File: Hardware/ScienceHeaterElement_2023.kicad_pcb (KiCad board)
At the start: 2 copper layers, 61.3 x 44.1 mm, 16 parts, among them Q1 BUK7M6R3-40EX, U1 LMT85DCK

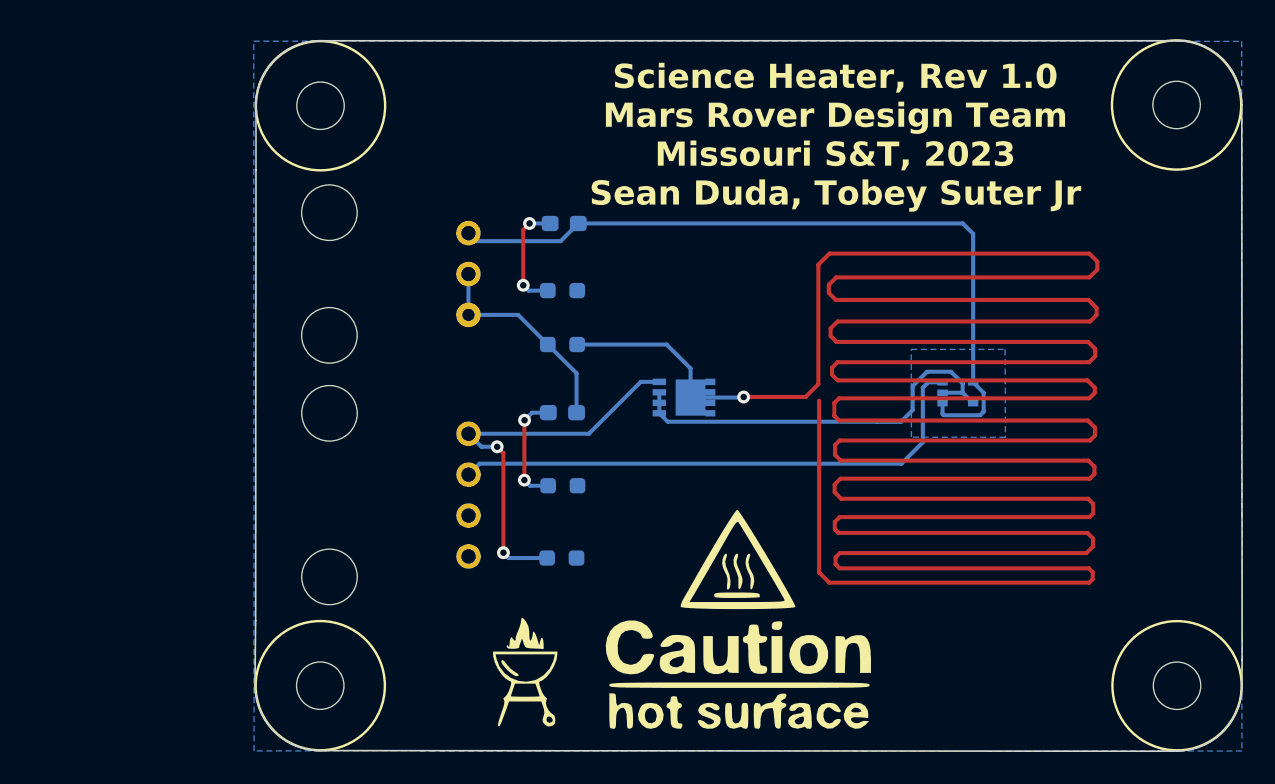
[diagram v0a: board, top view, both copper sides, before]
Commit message: Updated layout for order
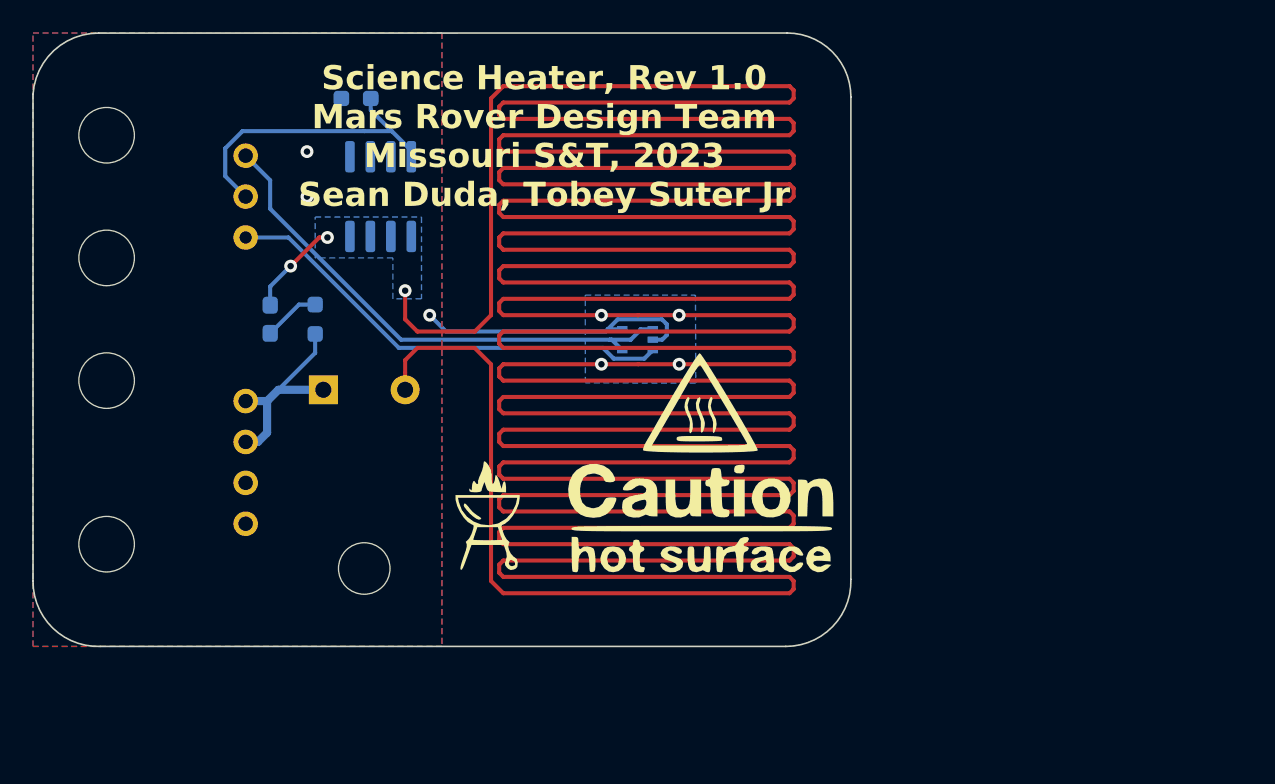
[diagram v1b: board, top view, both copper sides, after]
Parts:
- removed D2: Green, LED_SMD:LED_0603_1608Metric_Pad1.05x0.95mm_HandSolder
- removed R4: 4.7k, Resistor_SMD:R_0603_1608Metric_Pad0.98x0.95mm_HandSolder
- removed REF** (x4): 4_40_Hole, MRDT_Drill_Holes:4_40_Hole_Corner
- added G***: LOGO, LOGO, B.Cu at (105.2, 61.5)
- added G***: LOGO, LOGO, B.Cu at (91.9, 58.4)
- D1: value Green -> ORANGE
- Q1: value BUK7M6R3-40EX -> Si4162DY; footprint Package_TO_SOT_SMD:LFPAK33 -> Package_SO:SOIC-8_3.9x4.9mm_P1.27mm
- R1: value 2 -> 7.5; footprint Resistor_SMD:R_0603_1608Metric_Pad0.98x0.95mm_HandSolder -> Package_TO_SOT_THT:TO-126-2_Horizontal_TabDown
- R2: value 300 -> 1000
- R3: value 1k -> 4.7k
- moved R3 27.3 mm to (77.2, 35.8), turned to 180 degrees
- moved Q1 22.6 mm to (78.7, 41.9), turned to -90 degrees
- moved U1 20.2 mm to (94.7, 50.8), turned to 180 degrees
- moved D1 19.2 mm to (71.9, 49.5), turned to -90 degrees
- moved R2 15.5 mm to (74.7, 49.5), turned to 90 degrees
- moved R1 15.1 mm to (75.2, 53.9)
- moved Conn1 14.7 mm to (70.4, 39.4)
- moved Conn2 14.0 mm to (70.4, 54.6)
- moved G*** 10.00 mm to (98.6, 58.4)
- moved G*** 10.00 mm to (85.3, 61.5)
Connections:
- Conn1 pad 2: +12V -> Gate_Driving_Pin
- Conn1 pad 3: +12V -> Temp_Sense
- Conn2 pad 1: Gate_Driving_Pin -> +12V
- Conn2 pad 2: Temp_Sense -> +12V
- D1 pad 1: Net-(D1-K) -> /Heater_Trace
- D1 pad 2: +3.3V -> Net-(D1-A)
- R2 pad 1: Net-(D1-K) -> +12V
- R2 pad 2: GND -> Net-(D1-A)
- R3 pad 1: Net-(D2-K) -> Gate_Driving_Pin
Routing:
- net /Heater_Trace: track 343.9 -> 657.8 mm, vias 1 -> 7
- net +3.3V: track 47.0 -> 32.4 mm
- net GND: track 25.6 -> 18.1 mm, vias 0 -> 3
- net Net-(D2-K): track 7.02 -> 0.00 mm, vias 2 -> 0
- net Net-(D1-K): track 6.94 -> 0.00 mm, vias 2 -> 0
- net Gate_Driving_Pin: track 24.9 -> 19.0 mm, vias 2 -> 0
- net Temp_Sense: track 33.8 -> 28.6 mm
- net Net-(D1-A): track 0.00 -> 3.53 mm
- added copper zone on F.Cu, net GND
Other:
- board size 61.3 x 44.1 mm -> 50.8 x 38.1 mm
